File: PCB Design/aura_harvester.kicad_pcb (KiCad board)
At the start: 2 copper layers, 34.3 x 21.1 mm, 34 parts, among them J1 Conn_01x01_Pin, J2 Conn_01x01_Pin, J3 Conn_01x01_Pin, J4 Conn_01x01_Pin, J5 Conn_01x01_Pin, U1 ADG936BRUZ

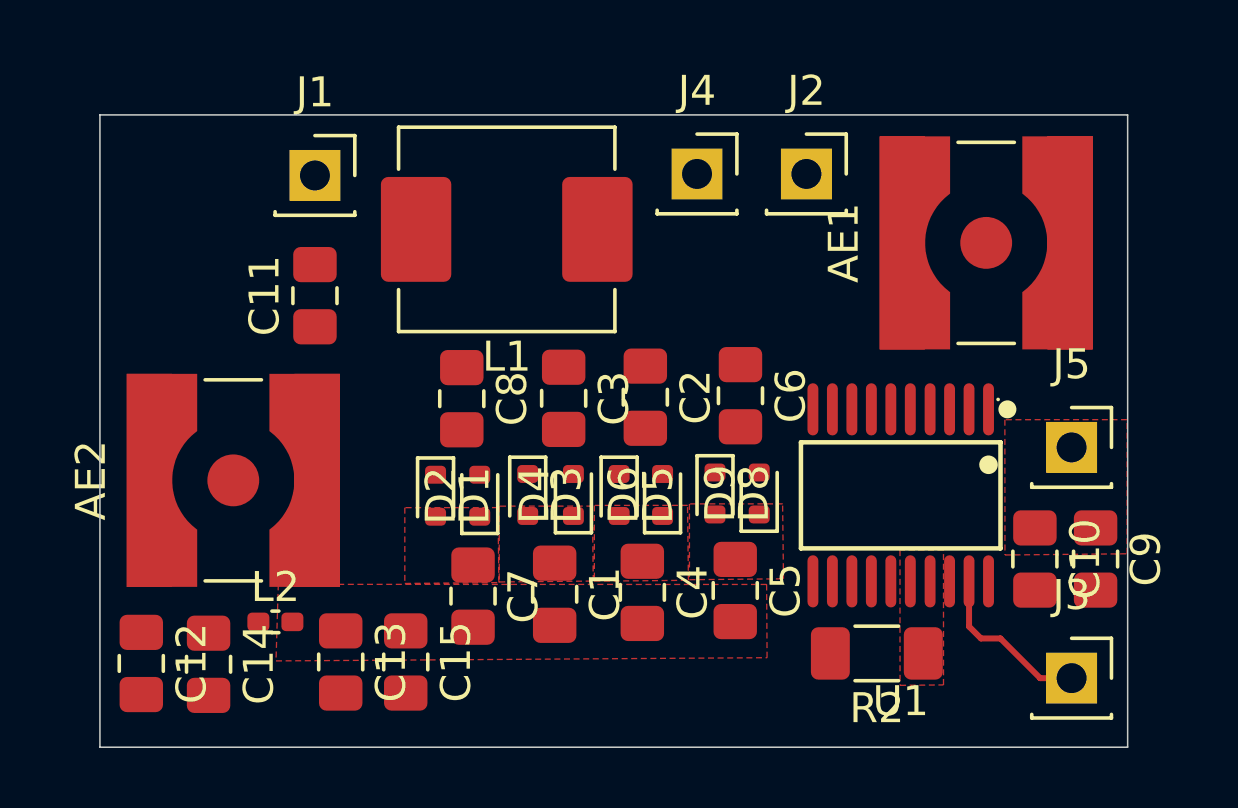
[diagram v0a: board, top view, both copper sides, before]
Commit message: Completed Routing and Silkscreen
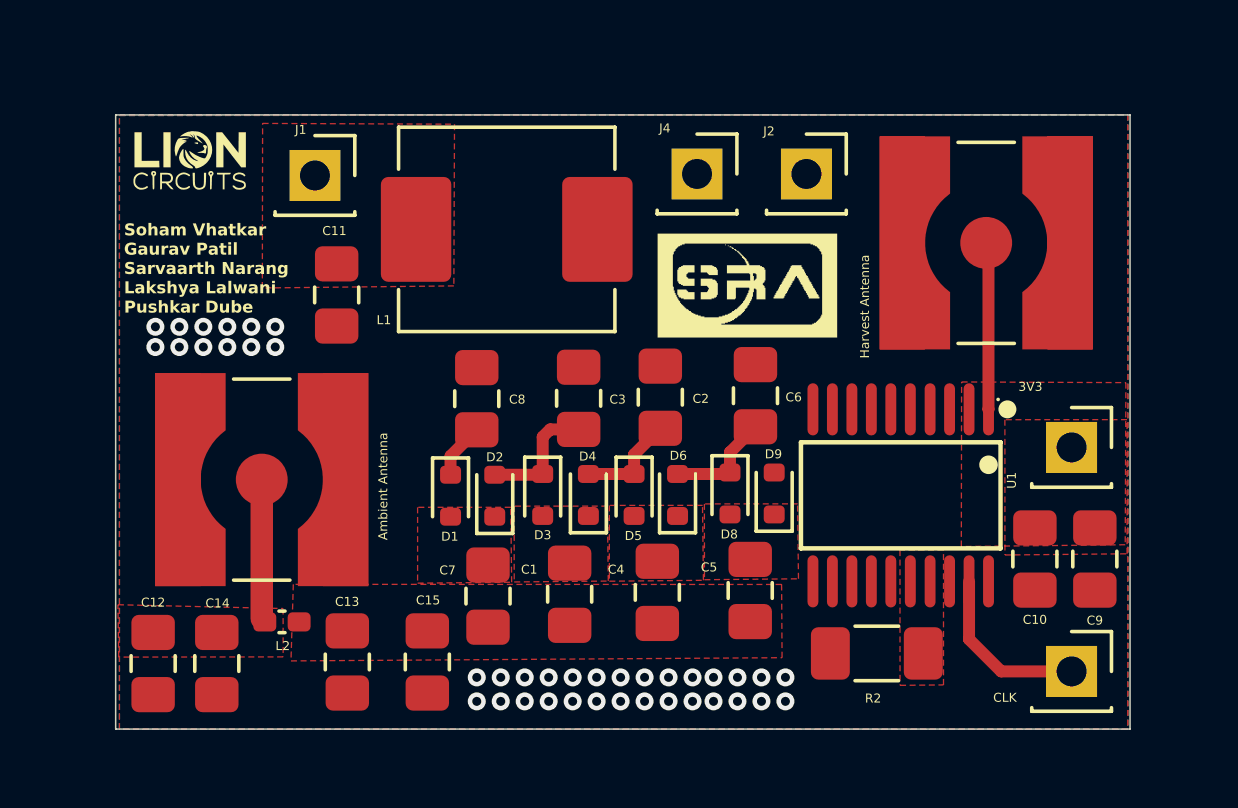
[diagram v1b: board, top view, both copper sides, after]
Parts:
- added G***: LOGO, Logos:Lions_logo, F.Cu at (60.0, 47.3)
- added G***: LOGO, logos:sra_logo_small_neg, F.Cu at (78.6, 51.5)
- Ambient Antenna: renamed from AE2
- Harvest Antenna: renamed from AE1
- L2: footprint Capacitor_SMD:C_0402_1005Metric_Pad0.74x0.62mm_HandSolder -> Inductor_SMD:L_0402_1005Metric_Pad0.77x0.64mm_HandSolder
- moved Ambient Antenna 0.95 mm to (62.4, 58.0)
- moved C11 0.73 mm to (64.9, 51.8)
- moved C15 0.72 mm to (67.9, 64.0)
- moved C1 0.50 mm to (72.7, 61.8)
- moved C2 0.50 mm to (75.7, 55.2)
- moved C3 0.50 mm to (73.0, 55.2)
- moved C4 0.50 mm to (75.6, 61.7)
- moved C5 0.50 mm to (78.7, 61.6)
- moved C6 0.50 mm to (78.8, 55.1)
- moved C7 0.50 mm to (69.9, 61.8)
- moved C8 0.50 mm to (69.5, 55.2)
- moved D1 0.50 mm to (68.7, 58.5)
- moved D2 0.50 mm to (70.2, 58.5)
- moved D3 0.50 mm to (71.8, 58.5)
- moved D4 0.50 mm to (73.3, 58.5)
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- renumbered J5 to 3V3, J3 to CLK
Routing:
- net /SMA_Sig: track 0.00 -> 5.59 mm
- net /Ambient_Source: track 0.00 -> 4.64 mm
- net Net-(D2-A): track 0.00 -> 4.15 mm
- net Net-(D6-A): track 0.00 -> 3.65 mm
- net Net-(D4-A): track 0.00 -> 3.41 mm
- net Net-(D1-K): track 0.00 -> 1.86 mm
- net GND: vias 0 -> 40
- added copper zone on F.Cu, net /Ambient_Source
- added copper zone on F.Cu, net /M_OUT
- added copper zone on B.Cu, net GND
- added copper zone on F.Cu, net GND
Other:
- board size 34.3 x 21.1 mm -> 33.8 x 20.5 mm
- board text added: "Soham Vhatkar Gaurav Patil Sarvaarth Narang Lakshya Lalwani Pushkar Dube"
